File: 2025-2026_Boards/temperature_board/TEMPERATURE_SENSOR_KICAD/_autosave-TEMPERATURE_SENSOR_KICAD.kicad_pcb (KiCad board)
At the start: 2 copper layers, 73.3 x 75.8 mm, 77 parts, among them J1 LCD Connector Pinout, J10 Conn_01x02_Pin, J11 Conn_01x02_Pin, J12 Conn_01x02_Pin, J13 Conn_01x02_Pin, J14 Conn_01x02_Pin, J15 Conn_01x02_Pin, J16 Conn_01x02_Pin, J17 Conn_01x02_Pin, J18 Conn_01x02_Pin, J19 Conn_01x02_Pin, J2 Conn_01x02_Pin, J20 Conn_01x02_Pin, J21 Conn_01x02_Pin, J22 Conn_01x02_Pin, J23 Conn_01x02_Pin, J24 Conn_01x03_Socket, J25 Conn_01x03_Socket, J3 Conn_01x02_Pin, J4 Conn_01x02_Pin, J5 Conn_01x02_Pin, J6 Conn_01x02_Pin, J7 Conn_01x02_Pin, J8 Conn_01x02_Pin, J9 Conn_01x02_Pin, U1 STM32G431CBT6, U2 TMP235A4DBZR, U3 AMS1117-3.3, U4 TCAN1057AEV-Q1, U5 TPS62932DRLR, U8 AMS1117

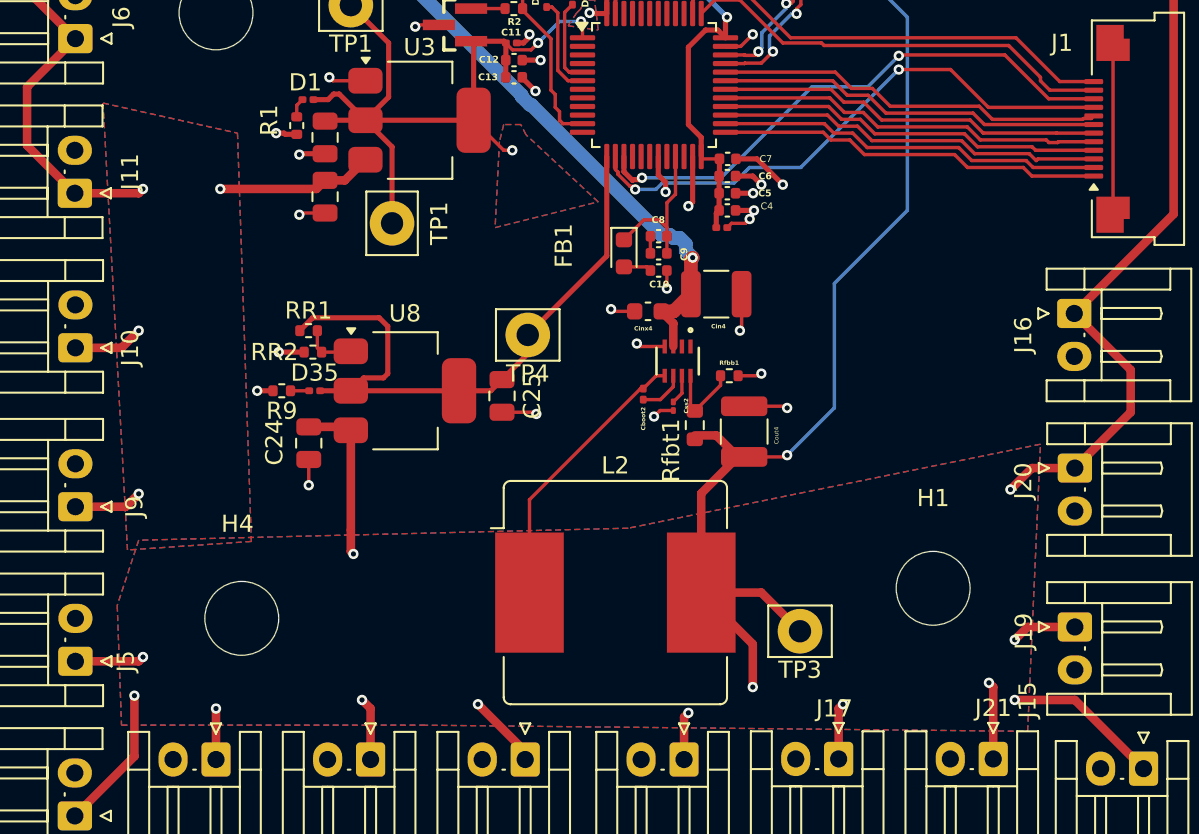
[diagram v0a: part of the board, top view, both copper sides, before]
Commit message: updates
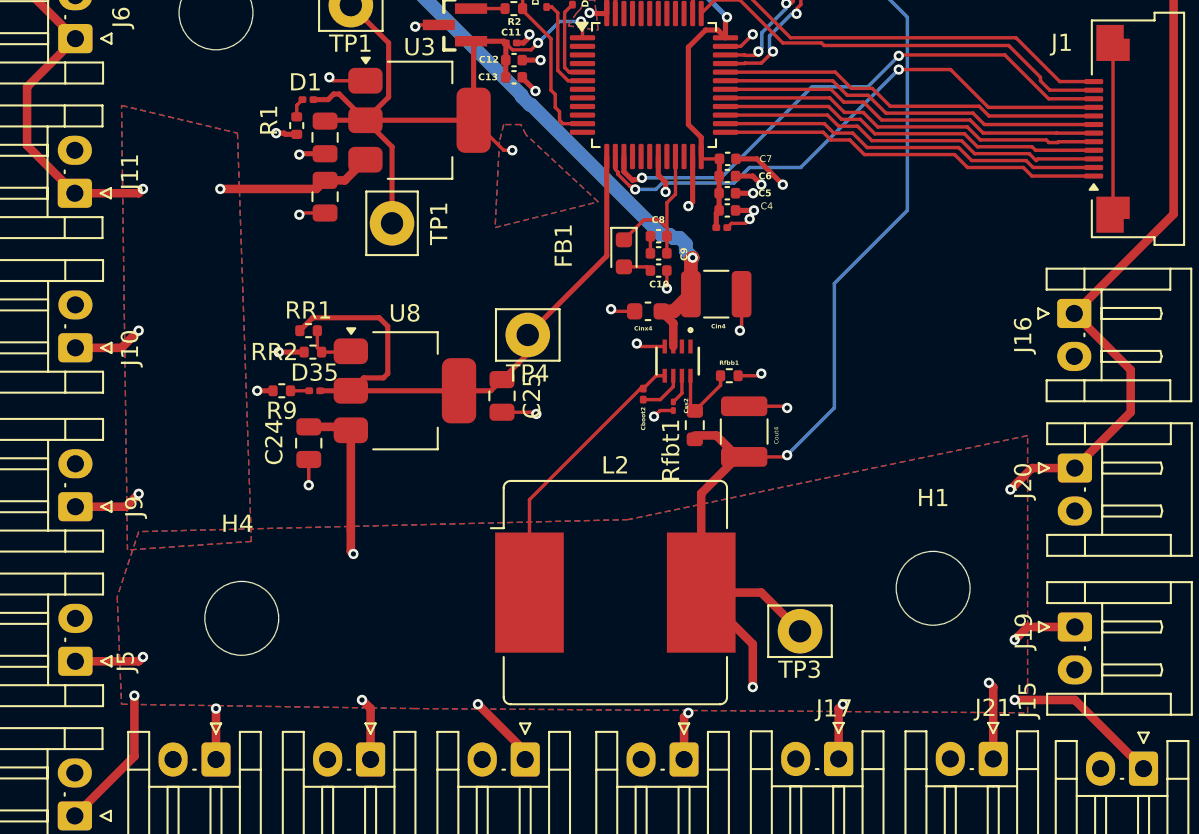
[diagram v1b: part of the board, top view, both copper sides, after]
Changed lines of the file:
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@@
 	)
 	(segment
-		(start 137.758598 125.899)
-		(end 138.201 125.899)
+		(start 132.25 125.75)
+		(end 138.35 125.75)
+		(width 0.2)
+		(layer "F.Cu")
+		(net 43)
+	)
+	(segment
+		(start 125.4604 124.14585)
+		(end 126.5 125.18545)
+		(width 0.2)
+		(layer "F.Cu")
+		(net 43)
+	)
+	(segment
+		(start 123.30415 123.2)
+		(end 124.25 124.14585)
+		(width 0.2)
+		(layer "F.Cu")
+		(net 43)
+	)
+	(segment
+		(start 131.68545 125.18545)
+		(end 132.25 125.75)
 		(width 0.2)
 		(layer "F.Cu")
@@
 	)
 	(segment
-		(start 131.68545 125.18545)
-		(end 132.449 125.949)
-		(width 0.2)
-		(layer "F.Cu")
-		(net 43)
-	)
-	(segment
-		(start 138.201 125.899)
-		(end 138.35 125.75)
-		(width 0.2)
-		(layer "F.Cu")
-		(net 43)
-	)
-	(segment
-		(start 132.449 125.949)
-		(end 137.708598 125.949)
-		(width 0.2)
-		(layer "F.Cu")
-		(net 43)
-	)
-	(segment
 		(start 126.5 125.18545)
 		(end 131.68545 125.18545)
-		(width 0.2)
-		(layer "F.Cu")
-		(net 43)
-	)
-	(segment
-		(start 125.4604 124.14585)
-		(end 126.5 125.18545)
-		(width 0.2)
-		(layer "F.Cu")
-		(net 43)
-	)
-	(segment
-		(start 137.708598 125.949)
-		(end 137.758598 125.899)
-		(width 0.2)
-		(layer "F.Cu")
-		(net 43)
-	)
-	(segment
-		(start 123.30415 123.2)
-		(end 124.25 124.14585)
 		(width 0.2)
 		(layer "F.Cu")
@@
 	)
 	(segment
+		(start 117.771802 114.16)
+		(end 118.375 113.556802)
+		(width 0.2)
+		(layer "F.Cu")
+		(net 48)
+	)
+	(segment
+		(start 116.575 113.75)
+		(end 116.985 114.16)
+		(width 0.2)
+		(layer "F.Cu")
+		(net 48)
+	)
+	(segment
+		(start 119.661647 110.025)
+		(end 119.318506 110.368141)
+		(width 0.2)
+		(layer "F.Cu")
+		(net 48)
+	)
+	(segment
+		(start 129 105.85)
+		(end 129.774999 106.624999)
+		(width 0.2)
+		(layer "F.Cu")
+		(net 48)
+	)
+	(segment
+		(start 117.6 108.475001)
+		(end 117.6 105.85)
+		(width 0.2)
+		(layer "F.Cu")
+		(net 48)
+	)
+	(segment
+		(start 115.9 113.75)
+		(end 116.575 113.75)
+		(width 0.2)
+		(layer "F.Cu")
+		(net 48)
+	)
+	(segment
+		(start 118.375 113.556802)
+		(end 118.375 109.250001)
+		(width 0.2)
+		(layer "F.Cu")
+		(net 48)
+	)
+	(segment
+		(start 129.774999 106.906803)
+		(end 126.656802 110.025)
+		(width 0.2)
+		(layer "F.Cu")
+		(net 48)
+	)
+	(segment
 		(start 126.656802 110.025)
 		(end 119.661647 110.025)
-		(width 0.2)
-		(layer "F.Cu")
-		(net 48)
-	)
-	(segment
-		(start 117.771802 114.16)
-		(end 118.375 113.556802)
-		(width 0.2)
-		(layer "F.Cu")
-		(net 48)
-	)
-	(segment
-		(start 116.575 113.75)
-		(end 116.985 114.16)
-		(width 0.2)
-		(layer "F.Cu")
-		(net 48)
-	)
-	(segment
-		(start 129 105.85)
-		(end 129.774999 106.624999)
-		(width 0.2)
-		(layer "F.Cu")
-		(net 48)
-	)
-	(segment
-		(start 129.774999 106.906803)
-		(end 126.656802 110.025)
-		(width 0.2)
-		(layer "F.Cu")
-		(net 48)
-	)
-	(segment
-		(start 117.6 108.475001)
-		(end 117.6 105.85)
-		(width 0.2)
-		(layer "F.Cu")
-		(net 48)
-	)
-	(segment
-		(start 115.9 113.75)
-		(end 116.575 113.75)
-		(width 0.2)
-		(layer "F.Cu")
-		(net 48)
-	)
-	(segment
-		(start 119.661647 110.025)
-		(end 119.318506 110.368141)
-		(width 0.2)
-		(layer "F.Cu")
-		(net 48)
-	)
-	(segment
-		(start 118.375 113.556802)
-		(end 118.375 109.250001)
 		(width 0.2)
 		(layer "F.Cu")
@@
 		(polygon
 			(pts
-				(xy 89.310399 150.521698) (xy 82.096668 151.019197) (xy 80.675 125) (xy 88.5 126.75)
+				(xy 89.310399 150.521698) (xy 82.096668 151.019197) (xy 81.75 125.14) (xy 88.5 126.75)
 			)
 		)
@@
 		(polygon
 			(pts
-				(xy 81.5 154.25) (xy 81.75 161.2175) (xy 99.25 161.2175) (xy 134.5 161.575) (xy 135.25 144.86) (xy 111.25 149.75)
-				(xy 82.75 150.45)
+				(xy 81.5 153.75) (xy 81.75 160) (xy 98.75 160.25) (xy 134.5 160.5) (xy 134.5 144.36) (xy 111.25 149.25)
+				(xy 82.75 149.95)
 			)
 		)
@@
 		(polygon
 			(pts
-				(xy 103.5 132.25) (xy 109.5 130.75) (xy 105.3 126.85) (xy 105 126.25) (xy 105 126.25) (xy 104 126.25)
-				(xy 103.75 127.25)
+				(xy 103.5 132.25) (xy 109.5 130.75) (xy 105.3 126.85) (xy 105 126.25) (xy 104 126.25) (xy 103.75 127.25)
 			)
 		)
